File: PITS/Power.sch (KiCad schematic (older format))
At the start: 22 parts, among them Q1 Q_PMOS_DGS, Q2 Q_PNP_dual, U5 LTC3112

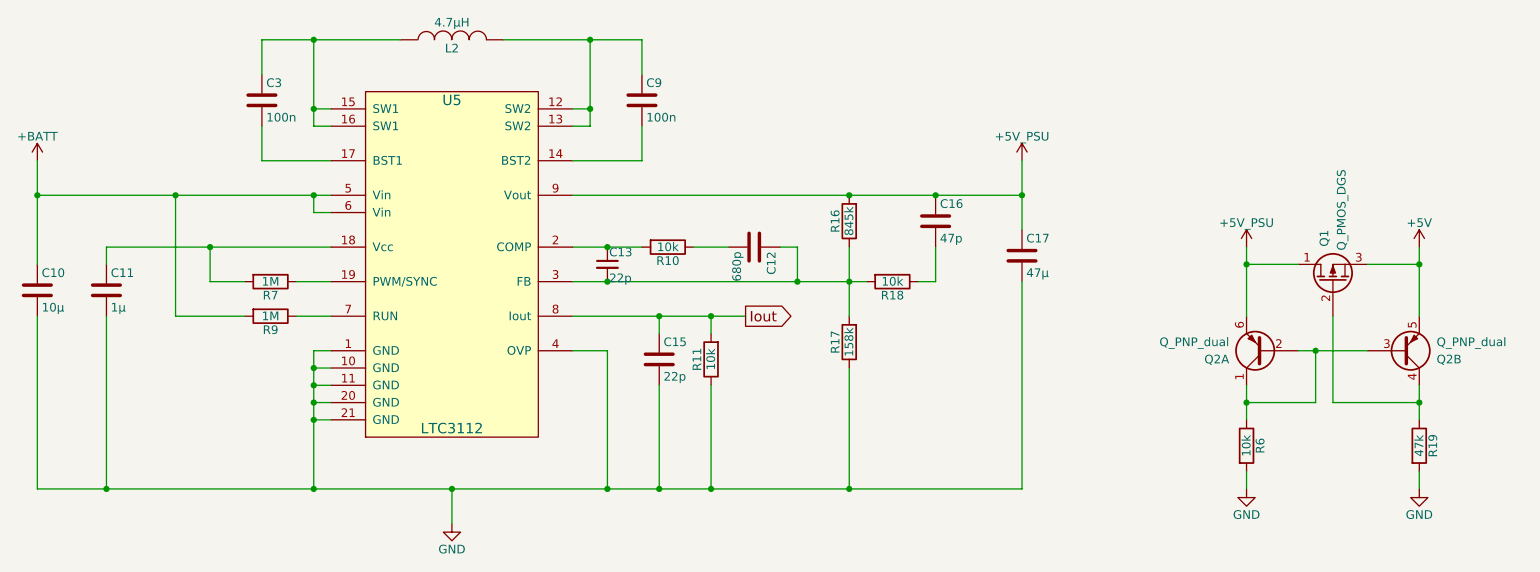
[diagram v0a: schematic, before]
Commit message: layout - work in progress
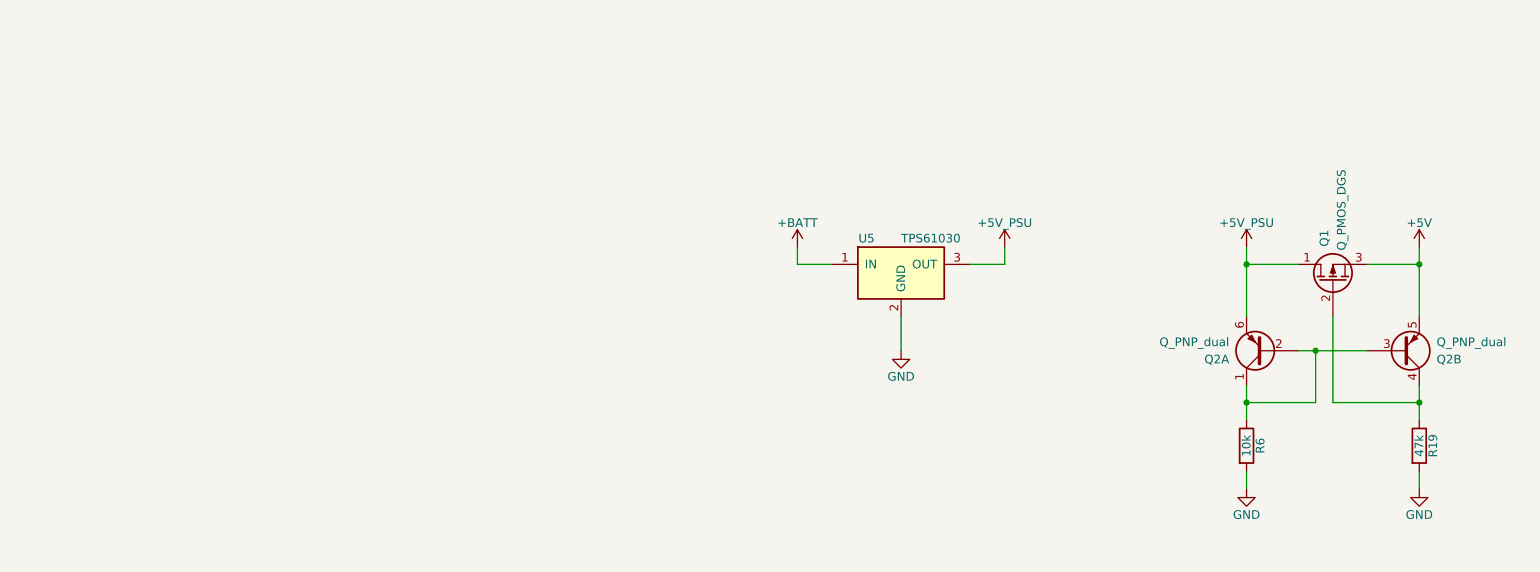
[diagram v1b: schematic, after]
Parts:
- removed C10: 10µ, Capacitors_SMD:C_1206_HandSoldering, symbol C
- removed C11: 1µ, Capacitors_SMD:C_0603_HandSoldering, symbol C
- removed C12: 680p, Capacitors_SMD:C_0603_HandSoldering, symbol C
- removed C13: 22p, Capacitors_SMD:C_0603_HandSoldering, symbol C_Small
- removed C15: 22p, Capacitors_SMD:C_0603_HandSoldering, symbol C
- removed C16: 47p, Capacitors_SMD:C_0603_HandSoldering, symbol C
- removed C17: 47µ, Capacitors_SMD:C_1206_HandSoldering, symbol C
- removed C3, C9: 100n, Capacitors_SMD:C_0603_HandSoldering, symbol C
- removed L2: 4.7µH, Inductors:Inductor_Wurth_HCI-7040, symbol INDUCTOR
- removed R10, R11, R18: 10k, Resistors_SMD:R_0603_HandSoldering, symbol R
- removed R16: 845k, Resistors_SMD:R_0603_HandSoldering, symbol R
- removed R17: 158k, Resistors_SMD:R_0603_HandSoldering, symbol R
- removed R7, R9: 1M, Resistors_SMD:R_0603_HandSoldering, symbol R
- removed U5: LTC3112, Housings_SSOP:ETSSOP-20-1EP_4.4x6.5mm_Pitch0.65mm, symbol LTC3112
- added U5: TPS61030, power:TPS61030, symbol LM7805CT
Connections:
- net +5V_PSU: now also U5.3 (OUT)
- net +BATT: now also U5.1 (IN)
- net GND: now also U5.2 (GND)
